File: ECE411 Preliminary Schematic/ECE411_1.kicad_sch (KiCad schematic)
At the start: 10 parts, among them J2 Raspberry_Pi_4, M1 Motor_Servo, U1 MCP3008

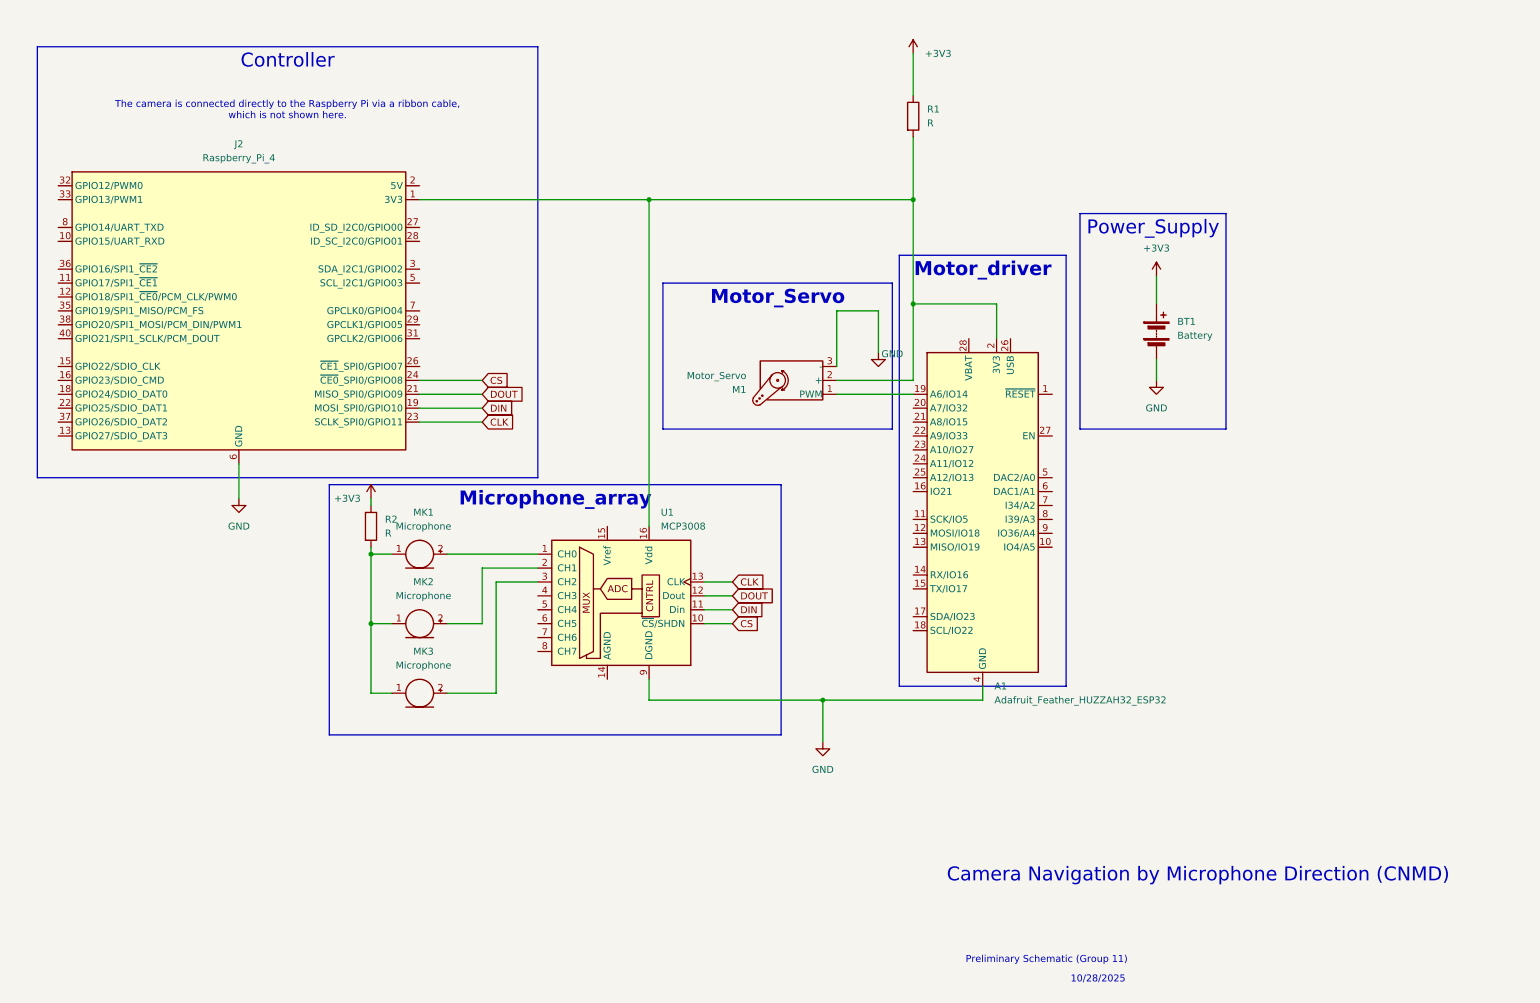
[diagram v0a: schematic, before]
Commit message: change the sch
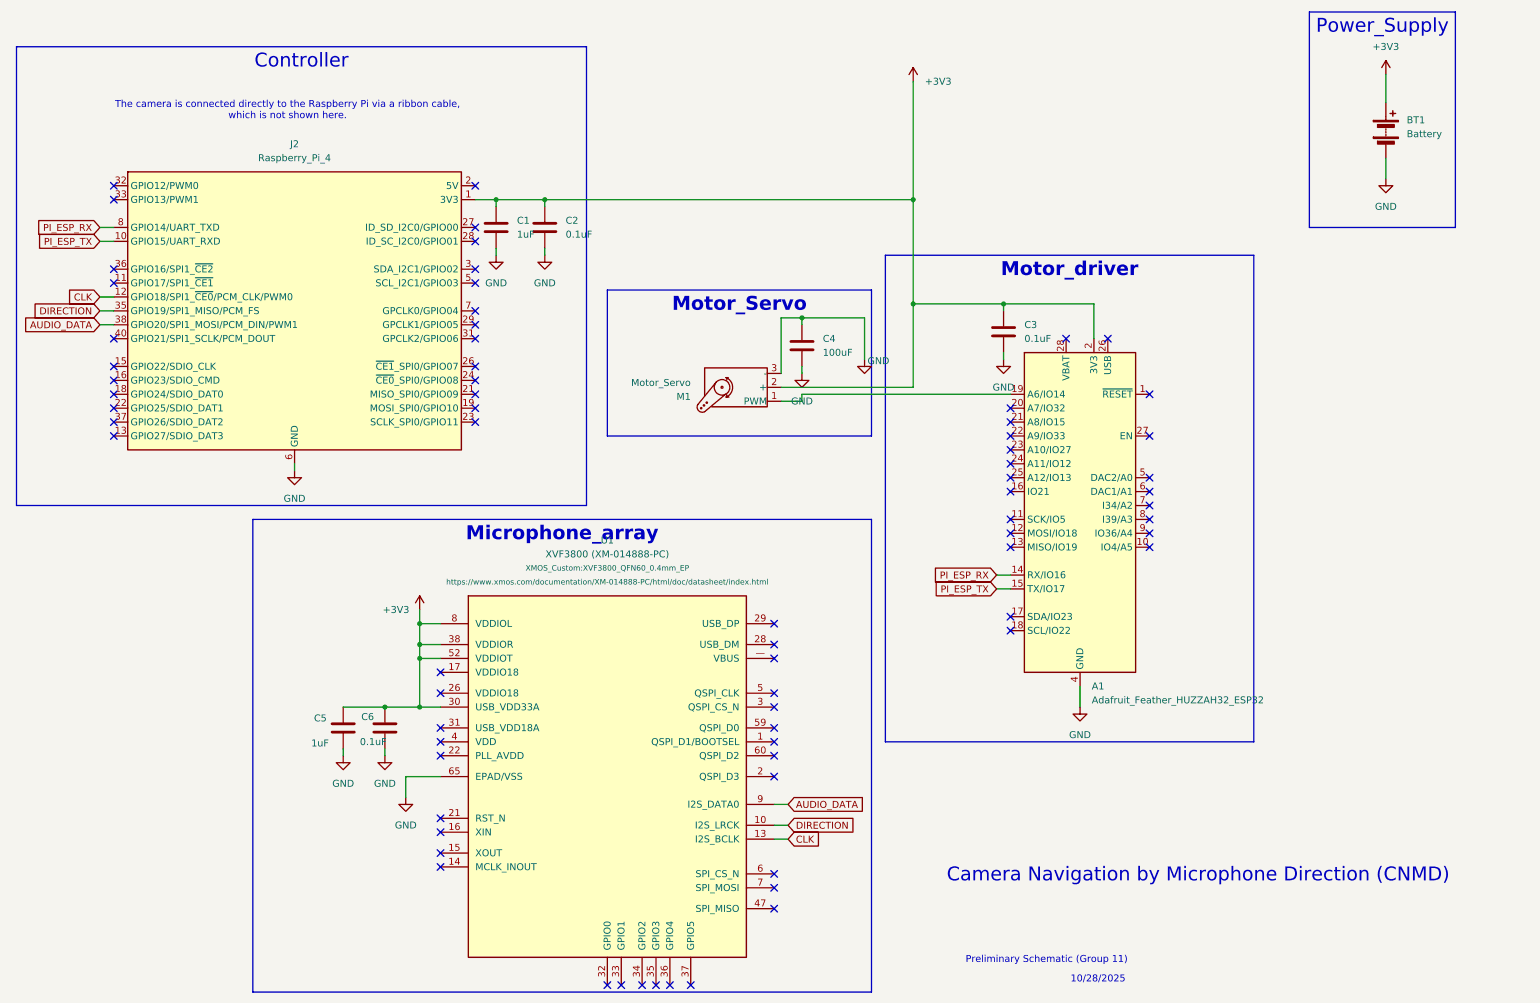
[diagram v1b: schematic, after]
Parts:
- removed MK1, MK2, MK3: Microphone, symbol Device:Microphone
- removed R1, R2: R, symbol Device:R
- removed U1: MCP3008, symbol Analog_ADC:MCP3008
- added C1, C5: 1uF, symbol Device:C
- added C2, C3, C6: 0.1uF, symbol Device:C
- added C4: 100uF, symbol Device:C
- added U1: XVF3800 (XM-014888-PC), XMOS_Custom:XVF3800_QFN60_0.4mm_EP, symbol XMOS_Custom:XVF3800
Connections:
- net +3V3: now also A1.2 (3V3), J2.1 (3V3), J2.17 (3V3), M1.2 (+), C1.1, C2.1, C3.1, C5.1, C6.1, U1.30 (USB_VDD33A), U1.38 (VDDIOR), U1.52 (VDDIOT), U1.8 (VDDIOL)
- net CLK: now also J2.12 (GPIO18/SPI1_~{CE0}/PCM_CLK/PWM0), U1.13 (I2S_BCLK); no longer J2.23 (SCLK_SPI0/GPIO11)
- net GND: now also C1.2, C2.2, C3.2, C4.1, C4.2, C5.2, C6.2, U1.65 (EPAD/VSS)
- net PI_ESP_RX: now reaches A1.14 (RX/IO16)
- net PI_ESP_RX: now also J2.8 (GPIO14/UART_TXD)
- net PI_ESP_TX: now reaches A1.15 (TX/IO17)
- net PI_ESP_TX: now also J2.10 (GPIO15/UART_RXD)
- net DIRECTION: now reaches J2.35 (GPIO19/SPI1_MISO/PCM_FS)
- net DIRECTION: now also U1.10 (I2S_LRCK)
- net AUDIO_DATA: now reaches J2.38 (GPIO20/SPI1_MOSI/PCM_DIN/PWM1)
- net AUDIO_DATA: now also U1.9 (I2S_DATA0)
- net CS: no longer names the net of J2.24 (~{CE0}_SPI0/GPIO08)
- net DIN: no longer names the net of J2.19 (MOSI_SPI0/GPIO10)
- net DOUT: no longer names the net of J2.21 (MISO_SPI0/GPIO09)
- no-connect marks 0 -> 73
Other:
- moved on the sheet: A1, BT1, J2, M1

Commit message: PCB draw ready
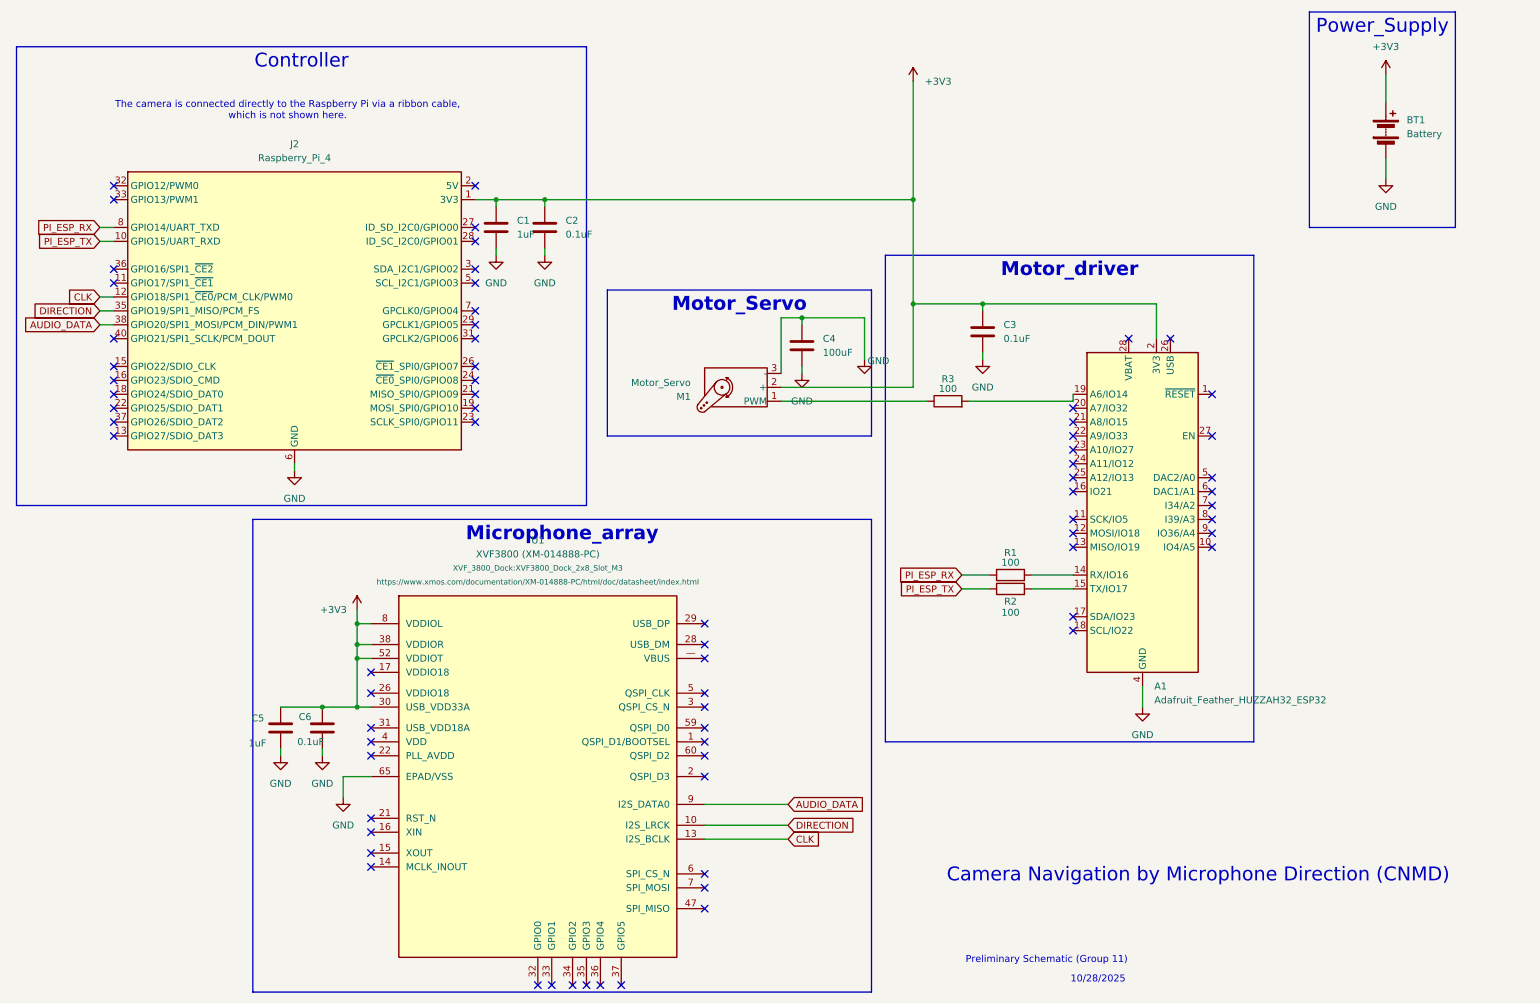
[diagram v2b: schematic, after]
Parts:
- added R1, R2, R3: 100, Resistor_SMD:R_0201_0603Metric, symbol Device:R
- BT1: footprint (none) -> Battery:BatteryHolder_Keystone_2462_2xAA
- C1, C2, C3, C4, C5, C6: footprint (none) -> Capacitor_SMD:C_0201_0603Metric
- J2: footprint (none) -> Module:Raspberry_Pi_Zero_Socketed_THT_FaceDown_MountingHoles
- M1: footprint (none) -> Connector_PinHeader_2.54mm:PinHeader_1x03_P2.54mm_Vertical
- U1: footprint XMOS_Custom:XVF3800_QFN60_0.4mm_EP -> XVF_3800_Dock:XVF3800_Dock_2x8_Slot_M3
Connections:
- net PI_ESP_RX: now also R1.1; no longer A1.14 (RX/IO16)
- net PI_ESP_TX: now also R2.1; no longer A1.15 (TX/IO17)
- net at A1.19 (A6/IO14): now also R3.2; no longer M1.1 (PWM)
- new net: A1.14 (RX/IO16), R1.2
- new net: A1.15 (TX/IO17), R2.2
- new net: M1.1 (PWM), R3.1
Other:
- moved on the sheet: A1, C3, C5, C6, U1
